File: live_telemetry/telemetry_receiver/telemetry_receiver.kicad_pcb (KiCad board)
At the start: 2 copper layers, 52.5 x 30.7 mm, 20 parts, among them J1 Conn_Coaxial, J2 Programming Header, J3 USB_A, U1 PIC16LF1455, U2 RFM95W, U3 AP2114H-3.3

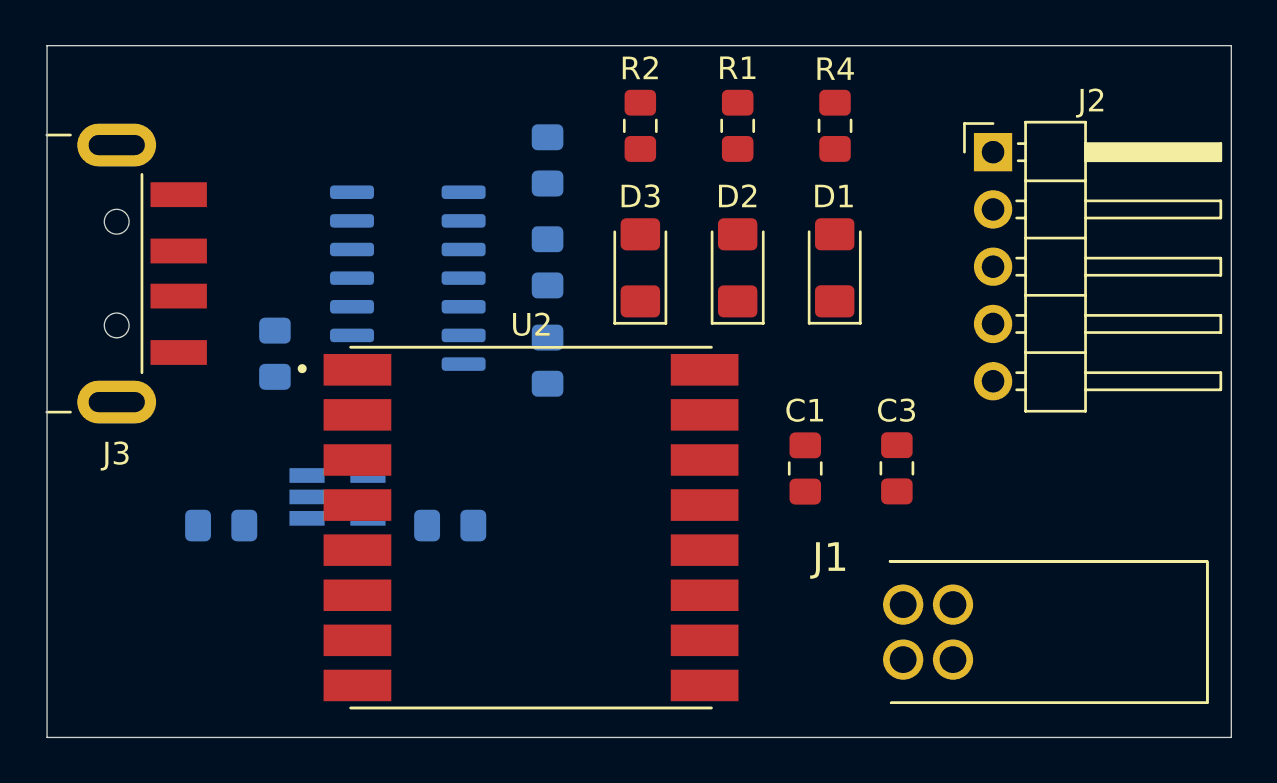
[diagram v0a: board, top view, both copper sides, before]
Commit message: Address Aaron's comments on initial component layout
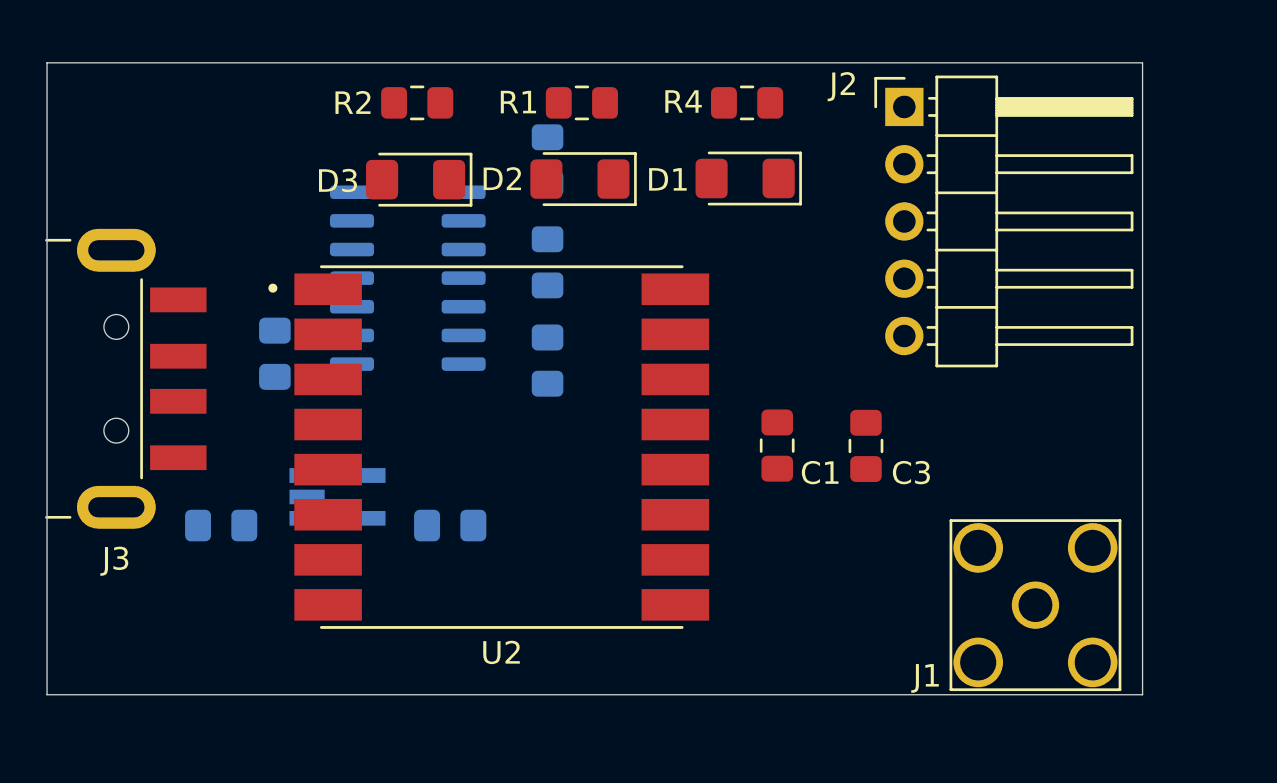
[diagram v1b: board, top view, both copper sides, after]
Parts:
- J1: footprint canhw_footprints:AmphenolRF_coaxial_conn_901-10510-2 -> canhw_footprints:RF_connector_SMA_3-1478978-1
- moved D3 10.7 mm to (124.3, 79.7), turned to 180 degrees
- moved R2 9.95 mm to (124.4, 76.3), turned to 180 degrees
- moved D2 8.03 mm to (131.6, 79.6), turned to 180 degrees
- moved R1 6.98 mm to (131.7, 76.3), turned to 180 degrees
- moved J1 5.87 mm to (151.8, 98.5)
- moved D1 5.61 mm to (138.9, 79.6), turned to 180 degrees
- moved J3 4.67 mm to (104.1, 88.5)
- moved J2 4.42 mm to (146.0, 76.4)
- moved R4 4.03 mm to (139.0, 76.3), turned to 180 degrees
- moved U2 3.80 mm to (128.1, 91.5)
- moved C3 1.69 mm to (144.3, 91.5)
- moved C1 1.61 mm to (140.3, 91.4)
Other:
- board size 52.5 x 30.7 mm -> 48.6 x 28 mm
